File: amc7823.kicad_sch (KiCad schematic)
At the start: 9 parts, among them U1301 AMC7823IRTAT

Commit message: fields
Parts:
- C1301, C1304, C1305: gfootprint 0402 -> (none)
- C1302, C1303, R1301, R1302, R1303: gfootprint 0603 -> (none)
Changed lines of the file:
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@@
-			)
-		)
-		(property "gfootprint" "0402"
-			(at 129.54 0 0)
-			(effects
-				(font
-					(size 1.27 1.27)
-				)
-				(hide yes)
 			)
 		)
@@
 			)
 		)
-		(property "gfootprint" "0603"
-			(at 0 101.6 0)
-			(effects
-				(font
-					(size 1.27 1.27)
-				)
-				(hide yes)
-			)
-		)
 		(pin "2"
 		)
@@
 			)
 		)
-		(property "gfootprint" "0603"
-			(at 335.28 335.28 0)
-			(effects
-				(font
-					(size 1.27 1.27)
-				)
-				(hide yes)
-			)
-		)
 		(pin "1"
 		)
@@
 			)
 		)
-		(property "gfootprint" "0603"
-			(at 0 116.84 0)
-			(effects
-				(font
-					(size 1.27 1.27)
-				)
-				(hide yes)
-			)
-		)
 		(pin "2"
 		)
@@
 			)
 		)
-		(property "gfootprint" "0603"
-			(at 161.29 161.29 0)
-			(effects
-				(font
-					(size 1.27 1.27)
-				)
-				(hide yes)
-			)
-		)
 		(pin "1"
 		)
@@
 			)
 		)
-		(property "gfootprint" "0402"
-			(at 434.34 0 0)
-			(effects
-				(font
-					(size 1.27 1.27)
-				)
-				(hide yes)
-			)
-		)
 		(pin "2"
 		)
@@
 			)
 		)
-		(property "gfootprint" "0402"
-			(at 0 101.6 0)
-			(effects
-				(font
-					(size 1.27 1.27)
-				)
-				(hide yes)
-			)
-		)
 		(pin "2"
 		)
@@
 			(effects
 				(font
-					(size 1.27 1.27)
-				)
-				(hide yes)
-			)
-		)
-		(property "gfootprint" "0603"
-			(at 10.16 -10.16 0)
-			(effects
-				(font

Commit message: vendor info
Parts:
- C1301, C1304, C1305: Vendor (none) -> digikey:490-1318-1-ND
- C1302, C1303: Vendor (none) -> digikey:490-3897-1-ND
- R1301, R1302, R1303: Vendor (none) -> digikey:311-4.75KHRCT-ND
- U1301: Vendor (none) -> digikey:296-18680-1-ND
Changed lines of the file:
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@@
+			)
+		)
+		(property "Vendor" "digikey:490-1318-1-ND"
+			(at 129.54 0 0)
+			(effects
+				(font
+					(size 1.27 1.27)
+				)
+				(hide yes)
 			)
 		)
@@
 			)
 		)
+		(property "Vendor" "digikey:490-3897-1-ND"
+			(at 0 101.6 0)
+			(effects
+				(font
+					(size 1.27 1.27)
+				)
+				(hide yes)
+			)
+		)
 		(pin "2"
 		)
@@
 			)
 		)
+		(property "Vendor" "digikey:311-4.75KHRCT-ND"
+			(at 335.28 335.28 0)
+			(effects
+				(font
+					(size 1.27 1.27)
+				)
+				(hide yes)
+			)
+		)
 		(pin "1"
 		)
@@
 			)
 		)
+		(property "Vendor" "digikey:490-3897-1-ND"
+			(at 0 116.84 0)
+			(effects
+				(font
+					(size 1.27 1.27)
+				)
+				(hide yes)
+			)
+		)
 		(pin "2"
 		)
@@
 			)
 		)
+		(property "Vendor" "digikey:296-18680-1-ND"
+			(at 0 165.1 0)
+			(effects
+				(font
+					(size 1.27 1.27)
+				)
+				(hide yes)
+			)
+		)
 		(pin "33"
 		)
@@
 			)
 		)
+		(property "Vendor" "digikey:311-4.75KHRCT-ND"
+			(at 161.29 161.29 0)
+			(effects
+				(font
+					(size 1.27 1.27)
+				)
+				(hide yes)
+			)
+		)
 		(pin "1"
 		)
@@
 			)
 		)
+		(property "Vendor" "digikey:490-1318-1-ND"
+			(at 434.34 0 0)
+			(effects
+				(font
+					(size 1.27 1.27)
+				)
+				(hide yes)
+			)
+		)
 		(pin "2"
 		)
@@
 			)
 		)
+		(property "Vendor" "digikey:490-1318-1-ND"
+			(at 0 101.6 0)
+			(effects
+				(font
+					(size 1.27 1.27)
+				)
+				(hide yes)
+			)
+		)
 		(pin "2"
 		)
@@
 			(effects
 				(font
+					(size 1.27 1.27)
+				)
+				(hide yes)
+			)
+		)
+		(property "Vendor" "digikey:311-4.75KHRCT-ND"
+			(at 10.16 -10.16 0)
+			(effects
+				(font

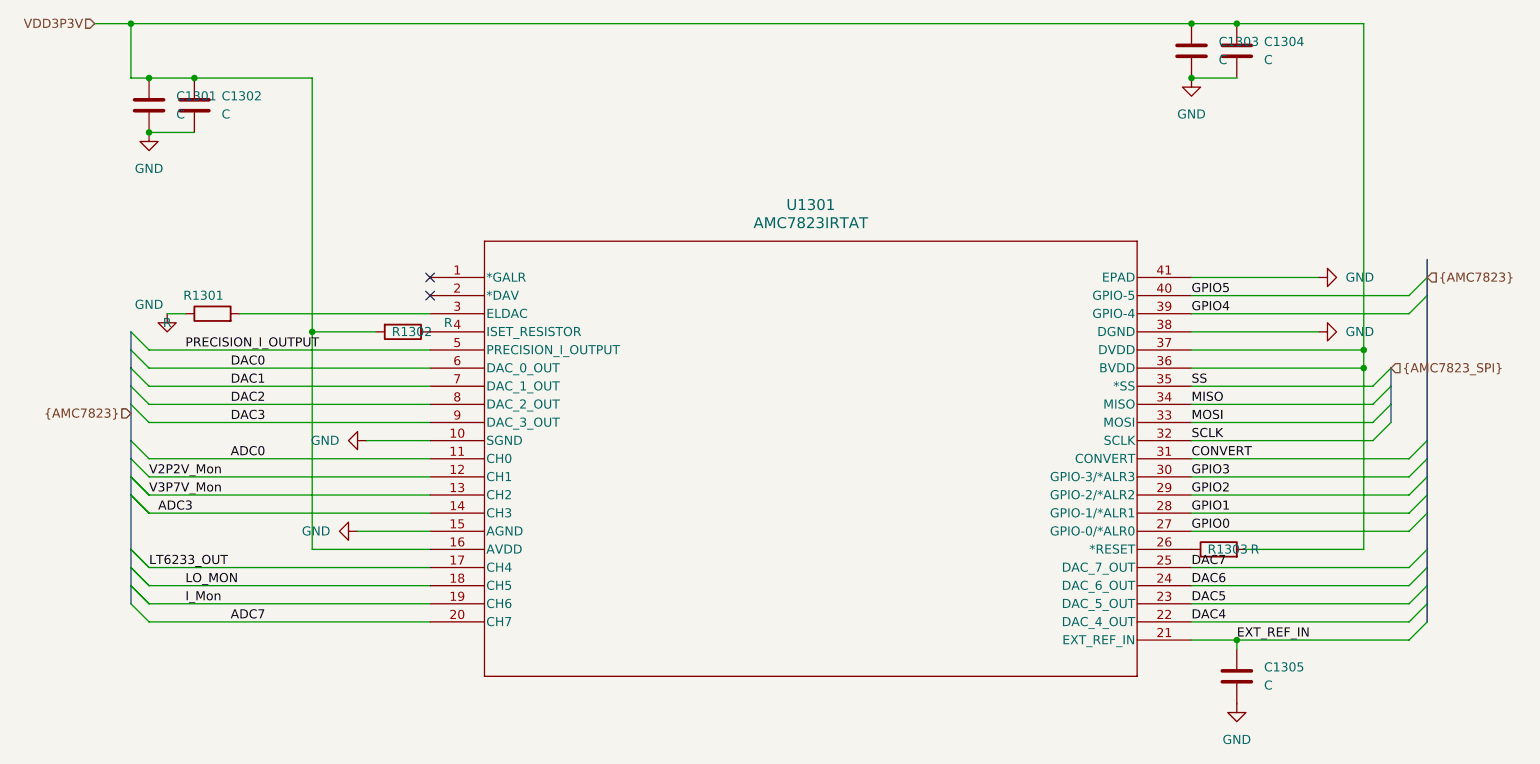
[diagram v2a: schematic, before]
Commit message: update value
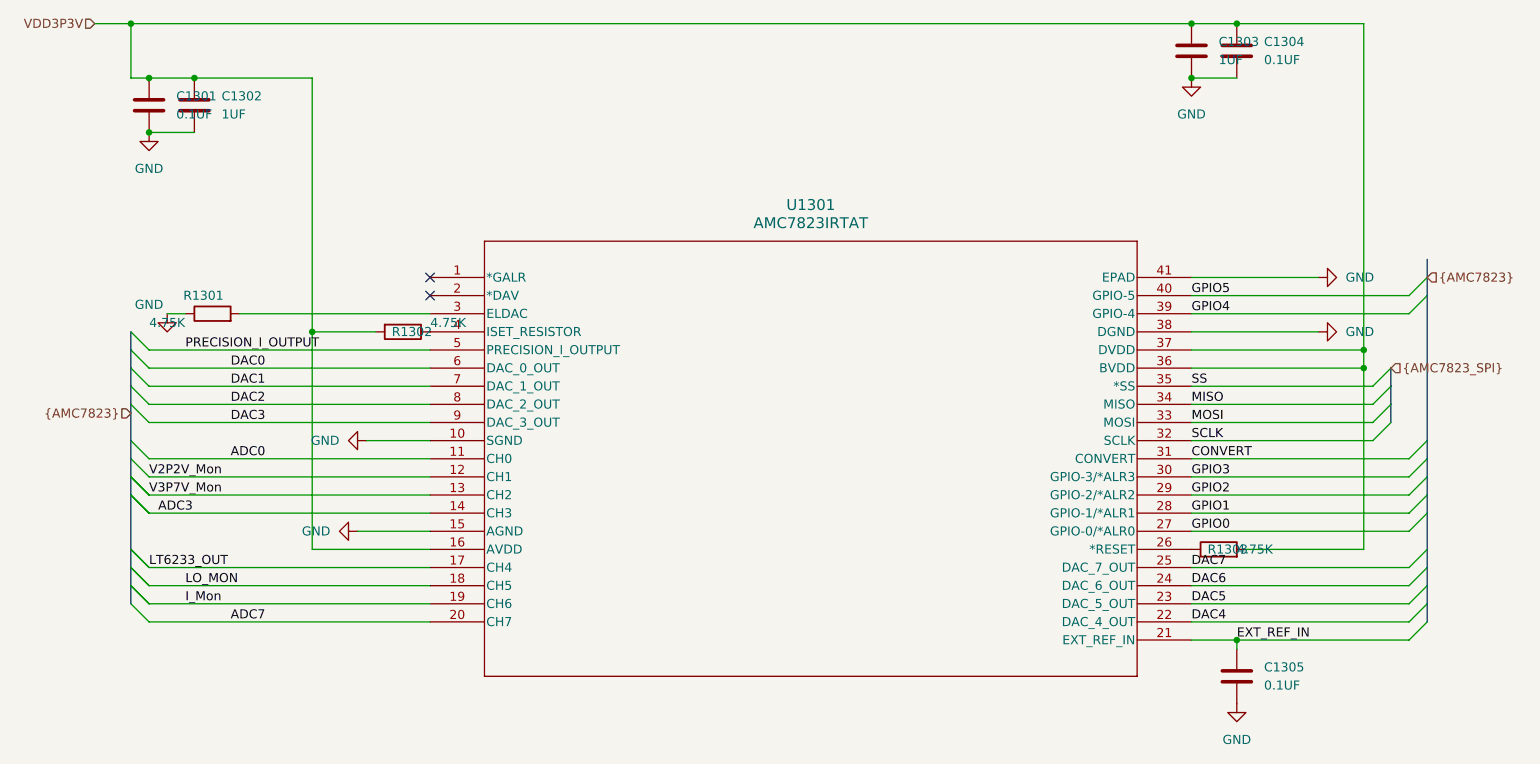
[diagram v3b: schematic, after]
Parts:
- C1301, C1304, C1305: value C -> 0.1UF
- C1302, C1303: value C -> 1UF
- R1301, R1302, R1303: value R -> 4.75K
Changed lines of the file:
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@@
 			)
 		)
-		(property "Value" "C"
+		(property "Value" "0.1UF"
 			(at 68.58 59.6899 0)
 			(effects
@@
 			)
 		)
-		(property "Value" "C"
+		(property "Value" "1UF"
 			(at 214.63 52.0699 0)
 			(effects
@@
 			)
 		)
-		(property "Value" "R"
+		(property "Value" "4.75K"
 			(at 219.71 120.65 90)
 			(effects
@@
 			)
 		)
-		(property "Value" "C"
+		(property "Value" "1UF"
 			(at 74.93 59.6899 0)
 			(effects
@@
 			)
 		)
-		(property "Value" "R"
+		(property "Value" "4.75K"
 			(at 67.31 88.9 90)
 			(effects
@@
 			)
 		)
-		(property "Value" "C"
+		(property "Value" "0.1UF"
 			(at 220.98 139.6999 0)
 			(effects
@@
 			)
 		)
-		(property "Value" "C"
+		(property "Value" "0.1UF"
 			(at 220.98 52.0699 0)
 			(effects
@@
 			)
 		)
-		(property "Value" "R"
+		(property "Value" "4.75K"
 			(at 106.68 88.9 90)
 			(effects
